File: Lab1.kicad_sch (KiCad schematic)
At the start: 15 parts, among them J1 Conn_02x05_Counter_Clockwise, SW1BOOT1 SW_Push, SW2NRST1 SW_Push, U1 STM32F407VGTx, Y1 Crystal

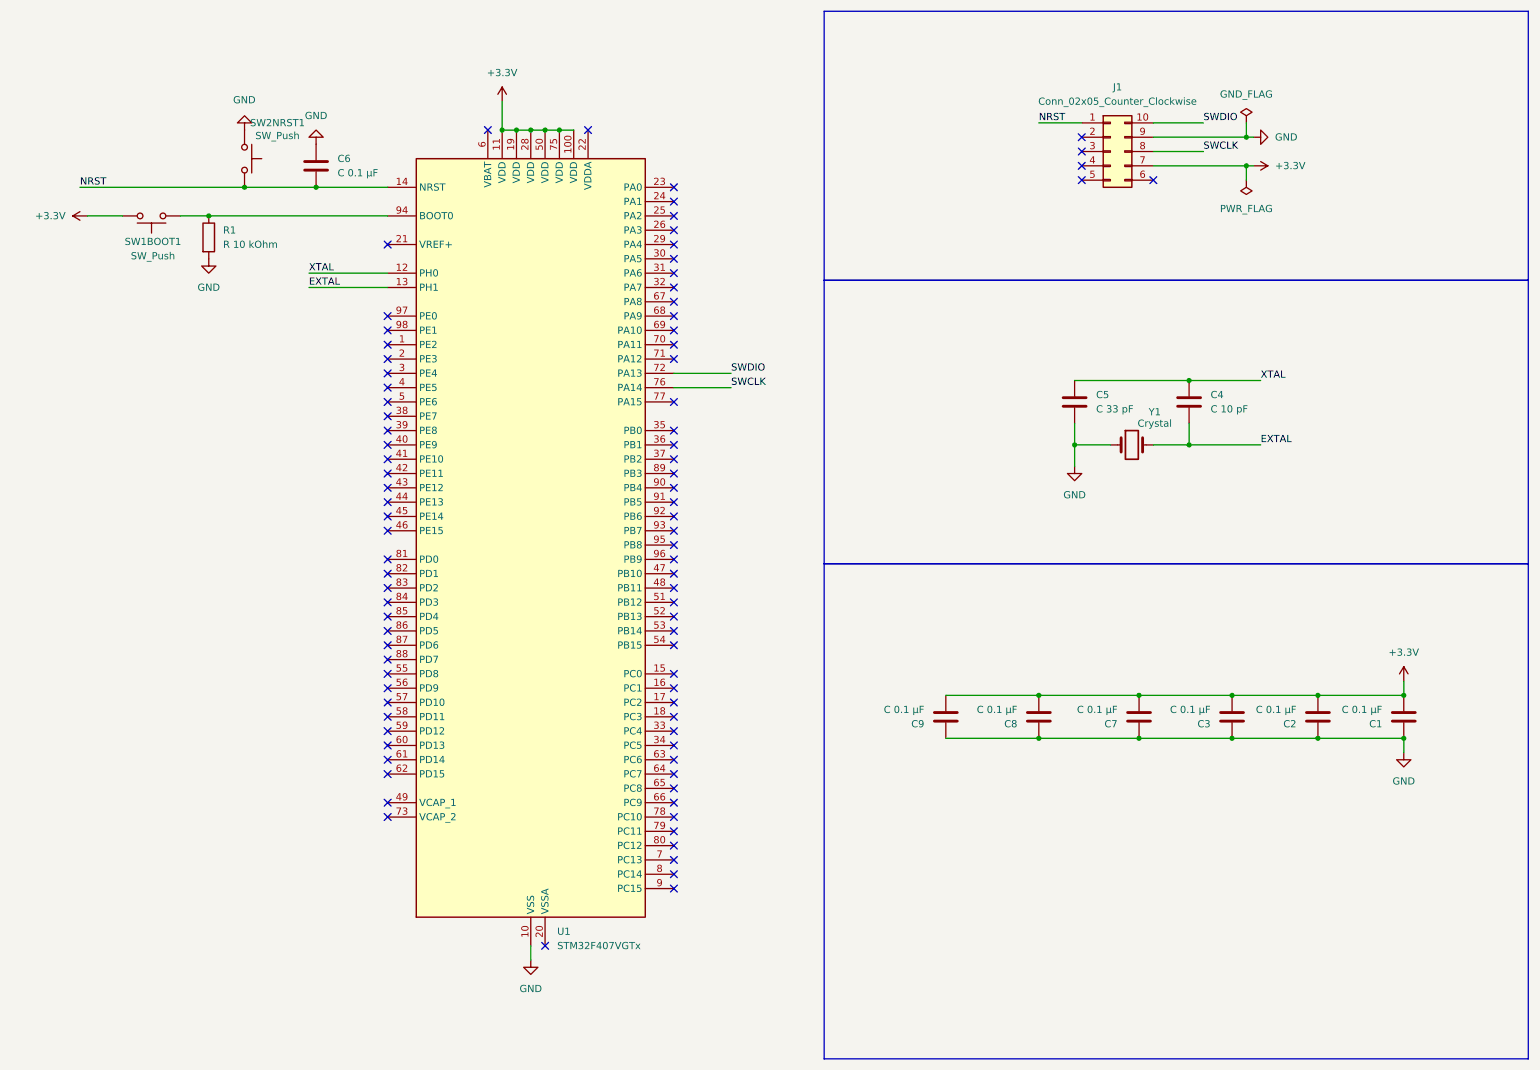
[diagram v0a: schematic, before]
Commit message: feat: add GPIO pins
feat: add user buttons

feat: add user LED

feat: add user potentiometer
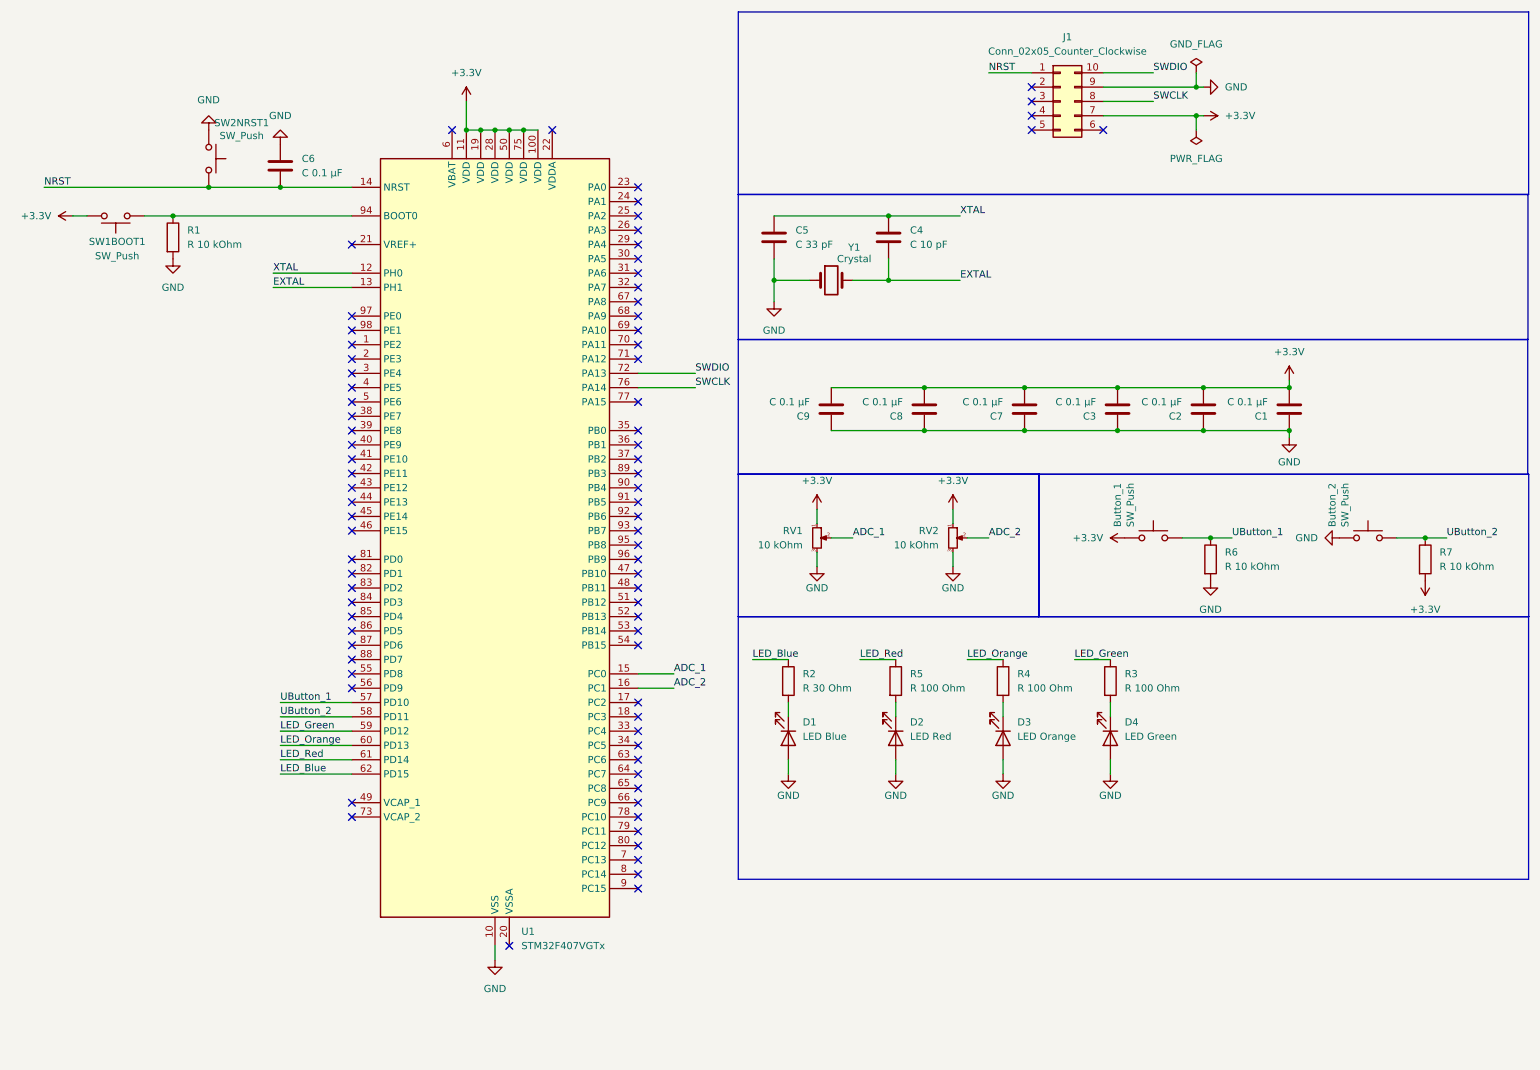
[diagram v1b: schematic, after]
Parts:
- added Button_1, Button_2: SW_Push, Button_Switch_THT:SW_PUSH_6mm, symbol Switch:SW_Push
- added D1: LED Blue, LED_SMD:LED_0805_2012Metric, symbol Device:LED
- added D2: LED Red, LED_SMD:LED_0805_2012Metric, symbol Device:LED
- added D3: LED Orange, LED_SMD:LED_0805_2012Metric, symbol Device:LED
- added D4: LED Green, LED_SMD:LED_0805_2012Metric, symbol Device:LED
- added R2: R 30 Ohm, Resistor_SMD:R_0805_2012Metric_Pad1.20x1.40mm_HandSolder, symbol Device:R
- added R3, R4, R5: R 100 Ohm, Resistor_SMD:R_0805_2012Metric_Pad1.20x1.40mm_HandSolder, symbol Device:R
- added R6, R7: R 10 kOhm, Resistor_SMD:R_0805_2012Metric_Pad1.20x1.40mm_HandSolder, symbol Device:R
- added RV1, RV2: 10 kOhm, Potentiometer_THT:Potentiometer_ACP_CA9-V10_Vertical, symbol Device:R_Potentiometer_Small
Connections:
- net +3.3V: now also Button_1.1, R7.2, RV1.1, RV2.1
- net GND: now also Button_2.1, D1.2 (A), D2.2 (A), D3.2 (A), D4.2 (A), R6.2, RV1.3, RV2.3
- net ADC_1: now reaches U1.15 (PC0)
- net ADC_1: now also RV1.2
- net ADC_2: now reaches U1.16 (PC1)
- net ADC_2: now also RV2.2
- net UButton_1: now reaches U1.57 (PD10)
- net UButton_1: now also Button_1.2, R6.1
- net UButton_2: now reaches U1.58 (PD11)
- net UButton_2: now also Button_2.2, R7.1
- net LED_Green: now reaches U1.59 (PD12)
- net LED_Green: now also R3.1
- net LED_Orange: now reaches U1.60 (PD13)
- net LED_Orange: now also R4.1
- net LED_Red: now reaches U1.61 (PD14)
- net LED_Red: now also R5.1
- net LED_Blue: now reaches U1.62 (PD15)
- net LED_Blue: now also R2.1
- new net: D2.1 (K), R5.2
- new net: D4.1 (K), R3.2
- new net: D1.1 (K), R2.2
- new net: D3.1 (K), R4.2
- no-connect marks 89 -> 81
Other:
- moved on the sheet: C1, C2, C3, C4, C5, C6, C7, C8, C9, J1, R1, SW1BOOT1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
